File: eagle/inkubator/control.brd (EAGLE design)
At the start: 100 x 80 mm, 29 parts, among them IC1 MEGA16-P, Q2 BS250, X1 USBPTH

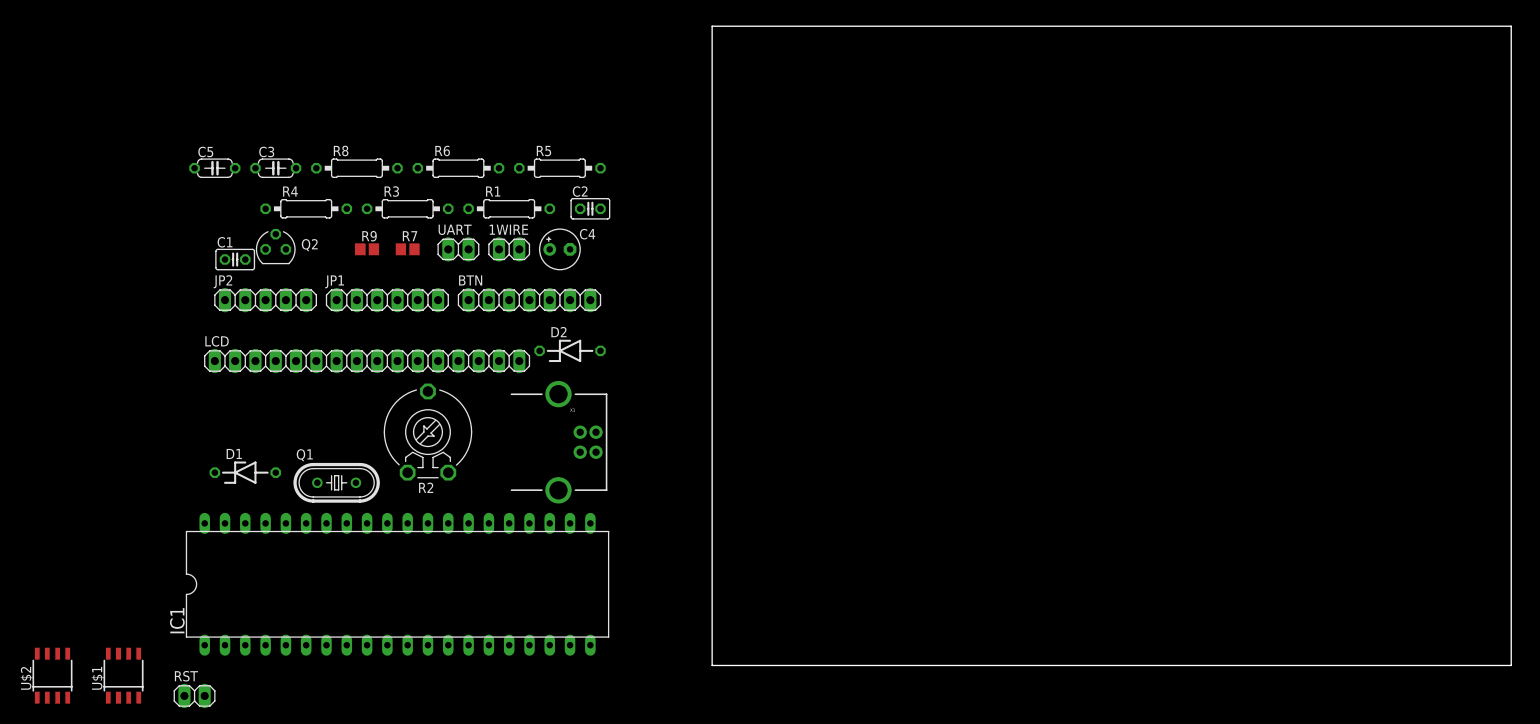
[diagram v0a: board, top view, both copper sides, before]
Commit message: schematic finished, board part 1
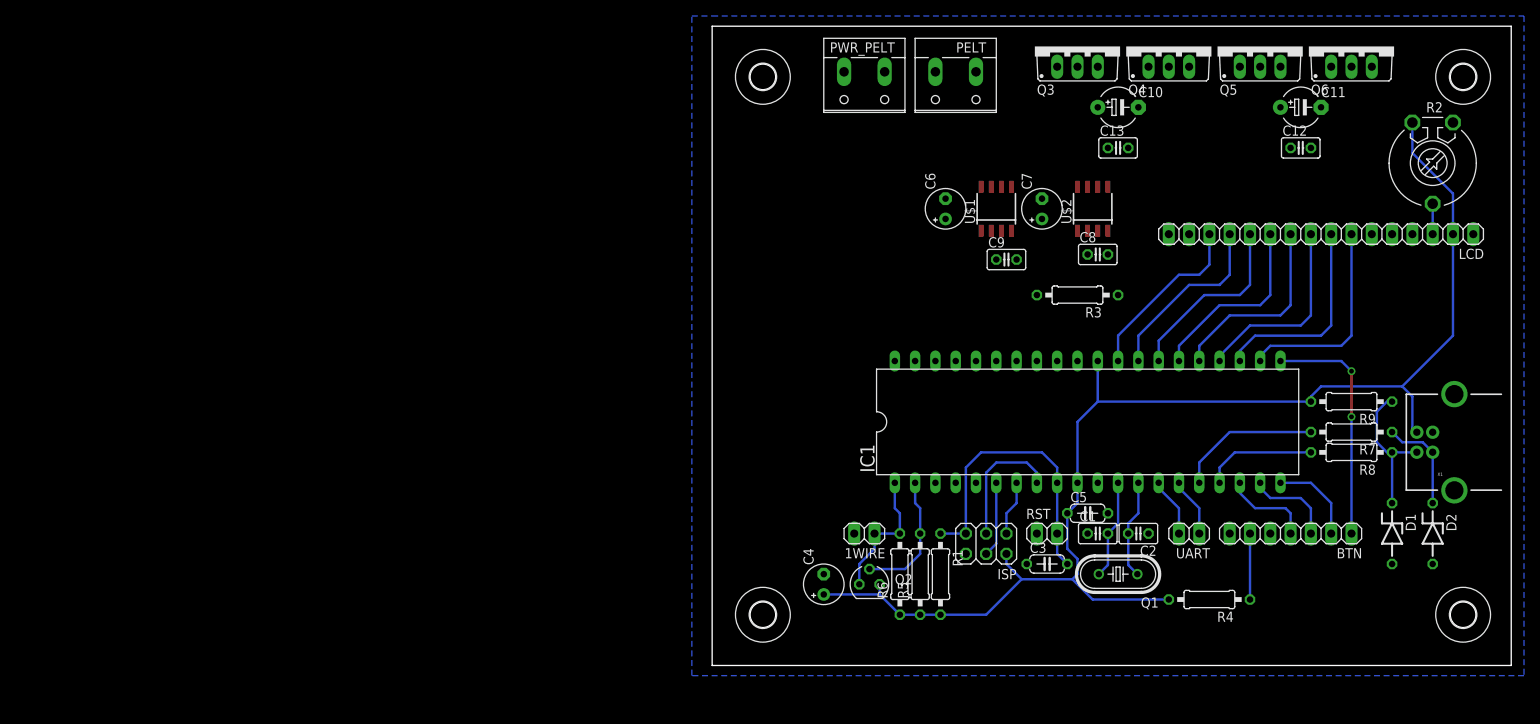
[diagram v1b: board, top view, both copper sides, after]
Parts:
- removed JP1: (no value), pinhead:1X06
- removed JP2: (no value), pinhead:1X05
- added C10, C11: 4u7, resistor:E5-5
- added C12, C13, C8, C9: 100n, resistor:C025-025X050
- added C6, C7: 10u, resistor:E2,5-5
- added H1, H2, H3, H4: MOUNT-HOLE3.2, holes:3,2
- added ISP: (no value), pinhead:2X03
- added PELT, PWR_PELT: (no value), con-wago-508:W237-132
- added Q3, Q4, Q5, Q6: IRF530, transistor-power:TO220BV
- R7, R9: device resistor:R0805 -> resistor:0207/10
- moved D1 143.7 mm to (85.1, 16.5), turned to 270 degrees
- moved U$2 142.7 mm to (47.6, 57.1)
- moved R2 130.2 mm to (90.2, 62.9), turned to 180 degrees
- moved R8 129.4 mm to (80.0, 26.7), turned to 180 degrees
- moved R9 124.7 mm to (80.0, 33.0), turned to 180 degrees
- moved U$1 123.9 mm to (35.6, 57.1)
- moved R4 123.2 mm to (62.2, 8.26), turned to 180 degrees
- moved LCD 120.4 mm to (76.2, 54.0), turned to 180 degrees
- moved R7 120.3 mm to (80.0, 29.2), turned to 180 degrees
- moved C5 117.4 mm to (47.0, 19.1)
- moved C1 113.3 mm to (48.3, 16.5)
- moved D2 110.3 mm to (90.2, 16.5), turned to 270 degrees
- moved RST 108.6 mm to (41.9, 16.5)
- moved C3 108.5 mm to (41.9, 12.7)
- moved X1 106.7 mm to (90.2, 27.9), turned to 180 degrees
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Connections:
- new net MISO: IC1.7, ISP.1
- new net MOSI: IC1.6, ISP.4
- new net N$41: Q5.G, U$2.3
- new net N$42: Q6.G, U$2.8
- new net N$46: C10.+, C11.+, C12.1, C13.1, PWR_PELT.2, Q3.D, Q5.D
- new net RESET: C3.2, IC1.9, ISP.5, R1.1, RST.2
- new net SCK: IC1.8, ISP.3
- net +5V: now also C6.+, C7.+, ISP.2, U$1.1, U$2.1
- net GND: now also C10.-, C11.-, C12.2, C13.2, C6.-, C7.-, ISP.6, PWR_PELT.1, Q4.S, Q6.S, U$1.7, U$2.7
- net N$3: now also IC1.33, U$2.5; no longer C3.2, IC1.9, R1.1, RST.2
- net N$30: now also IC1.34, U$2.6; no longer IC1.37, JP2.5
- net N$31: now also IC1.35, U$1.5; no longer IC1.36, JP2.4
- net N$32: now also IC1.36, U$1.6; no longer IC1.35, JP2.3
- net N$33: now also C9.1, U$1.2; no longer IC1.34, JP2.2
- net N$34: now also C8.1, U$2.2; no longer IC1.33, JP2.1
- net N$35: now also C8.2, U$2.4; no longer IC1.3, JP1.6
- net N$36: now also C9.2, U$1.4; no longer IC1.4, JP1.5
- net N$37: now also PELT.1, Q3.S, Q4.D; no longer IC1.5, JP1.4
- net N$38: now also PELT.2, Q5.S, Q6.D; no longer IC1.6, JP1.3
- net N$39: now also Q3.G, U$1.3; no longer IC1.7, JP1.2
- net N$40: now also Q4.G, U$1.8; no longer IC1.8, JP1.1
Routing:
- net +5V: track 0.00 -> 165.5 mm
- net RESET: track 0.00 -> 37.0 mm
- net N$21: track 0.00 -> 29.7 mm, vias 0 -> 2
- net N$7: track 0.00 -> 25.8 mm
- net N$8: track 0.00 -> 25.4 mm
- net N$9: track 0.00 -> 24.3 mm
- net N$10: track 0.00 -> 24.3 mm
- net N$11: track 0.00 -> 23.6 mm
- net N$12: track 0.00 -> 23.2 mm
- net N$13: track 0.00 -> 22.8 mm
- net N$14: track 0.00 -> 22.1 mm
- net N$29: track 0.00 -> 18.1 mm
- net N$18: track 0.00 -> 18.1 mm
- net N$25: track 0.00 -> 16.9 mm
- net N$4: track 0.00 -> 16.3 mm
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- added copper zone on layer 16, net GND
